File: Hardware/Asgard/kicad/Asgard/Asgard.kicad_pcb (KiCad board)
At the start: 2 copper layers, 17.8 x 61 mm, 9 parts

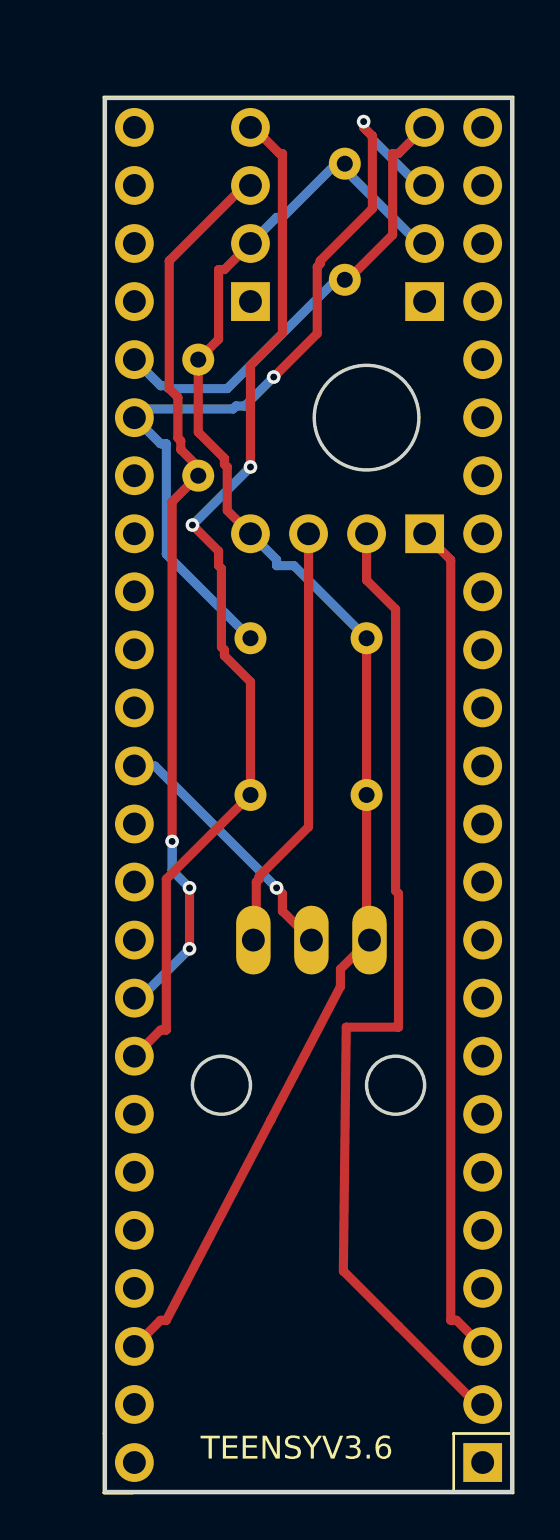
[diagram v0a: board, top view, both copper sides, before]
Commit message: PCB proposal
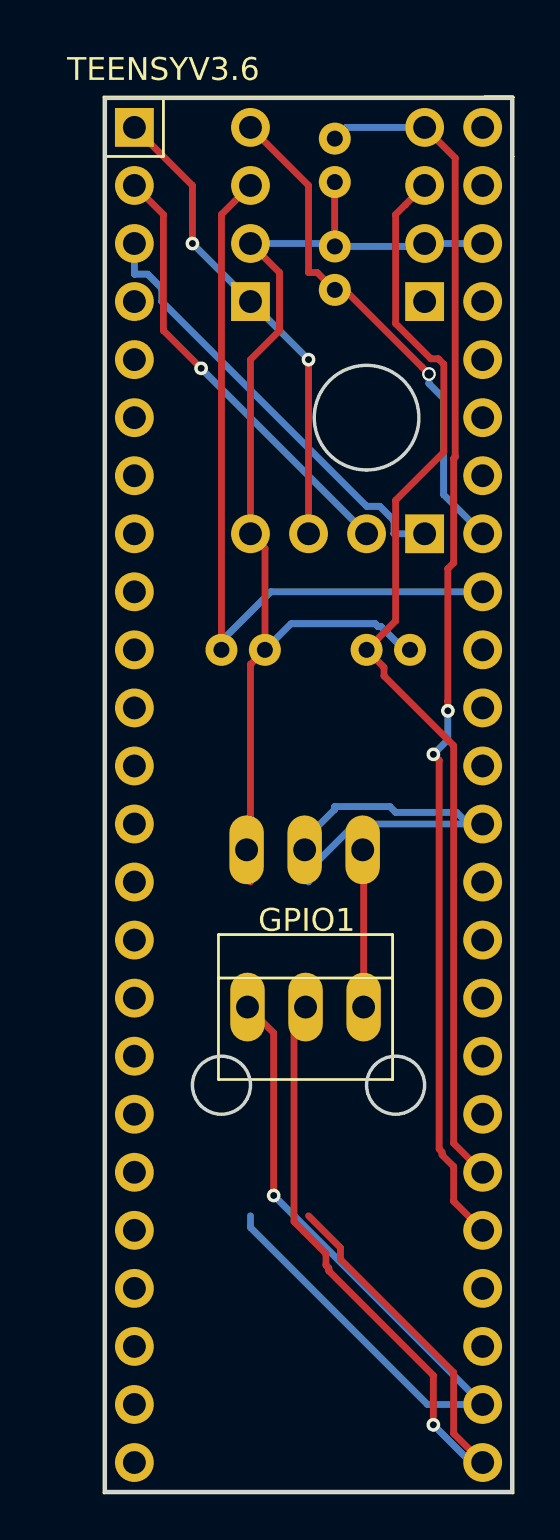
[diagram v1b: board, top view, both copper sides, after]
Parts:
- removed ABSP, BLUETOOTH, DELTAP: CONN_01X04, Socket_Strips:Socket_Strip_Straight_1x04_Pitch2.54mm
- removed OAT: CONN_01X03, Connect:PINHEAD1-3
- added ABSP1: CONN_01X04, Socket_Strips:Socket_Strip_Straight_1x04_Pitch2.54mm, B.Cu at (54.6, 39.4)
- added BLUETOOTH1: CONN_01X04, Socket_Strips:Socket_Strip_Straight_1x04_Pitch2.54mm, B.Cu at (54.6, 49.5)
- added DELTAP1: CONN_01X04, Socket_Strips:Socket_Strip_Straight_1x04_Pitch2.54mm, B.Cu at (47.0, 39.4)
- added GPIO1: CONN_01X03, Connect:PINHEAD1-3, F.Cu at (46.9, 70.2)
- added OAT1: CONN_01X03, Connect:PINHEAD1-3, B.Cu at (46.8, 63.4)
- R1, R2, R3, R4: footprint Resistors_THT:R_Axial_DIN0204_L3.6mm_D1.6mm_P5.08mm_Horizontal -> Resistors_ThroughHole:R_Axial_DIN0204_L3.6mm_D1.6mm_P1.90mm_Vertical
- moved TEENSYV3.6 58.4 mm to (49.5, 31.8), turned to 0 degrees
- moved R2 22.4 mm to (50.7, 38.9), turned to 90 degrees
- moved R1 7.69 mm to (45.7, 54.6), turned to 0 degrees
- moved R4 6.19 mm to (50.7, 32.2), turned to 270 degrees
- moved R3 5.11 mm to (52.1, 54.6)
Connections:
- TEENSYV3.6 pad 10: Net-(TEENSYV3.6-Pad10) -> (no net)
- TEENSYV3.6 pad 11: Net-(TEENSYV3.6-Pad11) -> (no net)
- TEENSYV3.6 pad 12: Net-(TEENSYV3.6-Pad12) -> (no net)
- TEENSYV3.6 pad 13: Net-(TEENSYV3.6-Pad13) -> (no net)
- TEENSYV3.6 pad 14: Net-(TEENSYV3.6-Pad14) -> (no net)
- TEENSYV3.6 pad 15: Net-(TEENSYV3.6-Pad15) -> (no net)
- TEENSYV3.6 pad 16: Net-(TEENSYV3.6-Pad16) -> (no net)
- TEENSYV3.6 pad 17: Net-(TEENSYV3.6-Pad17) -> (no net)
- TEENSYV3.6 pad 18: Net-(TEENSYV3.6-Pad18) -> (no net)
- TEENSYV3.6 pad 19: Net-(TEENSYV3.6-Pad19) -> (no net)
- TEENSYV3.6 pad 20: Net-(TEENSYV3.6-Pad20) -> (no net)
- TEENSYV3.6 pad 21: Net-(TEENSYV3.6-Pad21) -> (no net)
- TEENSYV3.6 pad 22: Net-(TEENSYV3.6-Pad22) -> (no net)
- TEENSYV3.6 pad 23: Net-(TEENSYV3.6-Pad23) -> (no net)
- TEENSYV3.6 pad 24: Net-(TEENSYV3.6-Pad24) -> (no net)
- TEENSYV3.6 pad 25: Net-(TEENSYV3.6-Pad25) -> (no net)
- TEENSYV3.6 pad 26: Net-(TEENSYV3.6-Pad26) -> (no net)
- TEENSYV3.6 pad 28: Net-(TEENSYV3.6-Pad28) -> (no net)
- TEENSYV3.6 pad 29: Net-(TEENSYV3.6-Pad29) -> (no net)
- TEENSYV3.6 pad 30: Net-(TEENSYV3.6-Pad30) -> (no net)
- TEENSYV3.6 pad 31: Net-(TEENSYV3.6-Pad31) -> (no net)
- TEENSYV3.6 pad 34: Net-(TEENSYV3.6-Pad34) -> (no net)
- TEENSYV3.6 pad 35: Net-(TEENSYV3.6-Pad35) -> (no net)
- TEENSYV3.6 pad 36: Net-(TEENSYV3.6-Pad36) -> (no net)
- TEENSYV3.6 pad 38: Net-(TEENSYV3.6-Pad38) -> (no net)
- TEENSYV3.6 pad 39: Net-(TEENSYV3.6-Pad39) -> (no net)
- TEENSYV3.6 pad 4: Net-(TEENSYV3.6-Pad4) -> (no net)
- TEENSYV3.6 pad 40: Net-(TEENSYV3.6-Pad40) -> (no net)
- TEENSYV3.6 pad 41: Net-(TEENSYV3.6-Pad41) -> (no net)
- TEENSYV3.6 pad 42: Net-(TEENSYV3.6-Pad42) -> (no net)
- TEENSYV3.6 pad 45: Net-(TEENSYV3.6-Pad45) -> (no net)
- TEENSYV3.6 pad 46: Net-(TEENSYV3.6-Pad46) -> (no net)
- TEENSYV3.6 pad 5: Net-(TEENSYV3.6-Pad5) -> (no net)
- TEENSYV3.6 pad 6: Net-(TEENSYV3.6-Pad6) -> (no net)
- TEENSYV3.6 pad 7: Net-(TEENSYV3.6-Pad7) -> (no net)
- TEENSYV3.6 pad 8: Net-(TEENSYV3.6-Pad8) -> (no net)
- TEENSYV3.6 pad 9: Net-(TEENSYV3.6-Pad9) -> (no net)
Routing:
- net Net-(GPIO1-Pad2): track 0.00 -> 37.8 mm, vias 0 -> 1
- net Net-(GPIO1-Pad1): track 0.00 -> 35.5 mm, vias 0 -> 1
- net Net-(ABSP1-Pad4): track 20.2 -> 54.3 mm, vias 0 -> 2
- net Net-(BLUETOOTH1-Pad2): track 43.6 -> 19.4 mm, vias 0 -> 1
- net Net-(DELTAP1-Pad4): track 46.3 -> 22.5 mm, vias 2 -> 1
- net Net-(BLUETOOTH1-Pad1): track 36.8 -> 19.4 mm
- net +3V3: track 66.8 -> 49.9 mm
- net GND: track 18.8 -> 33.4 mm, vias 0 -> 2
- net Net-(ABSP1-Pad3): track 35.9 -> 48.3 mm, vias 2 -> 0
- net Net-(DELTAP1-Pad3): track 39.6 -> 33.6 mm, vias 3 -> 0
- net Net-(OAT1-Pad2): track 11.3 -> 12.7 mm, vias 1 -> 0
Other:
- net class Default: clearance 0.3 -> 0.2; trace_width 0.4 -> 0.3
- rule trace_clearance: 0.3 -> 0.2
- rule trace_min: 0.4 -> 0.3
